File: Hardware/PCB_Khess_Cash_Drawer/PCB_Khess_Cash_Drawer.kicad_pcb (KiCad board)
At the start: 2 copper layers, 92 x 84 mm, 17 parts, among them J1 Screw_Terminal_01x02, J2 Conn_01x02, J3 RJ11_Connector, J4 USB3_A, Q1 BUK9637-100E,118, U1 R-78B5.0-2.0

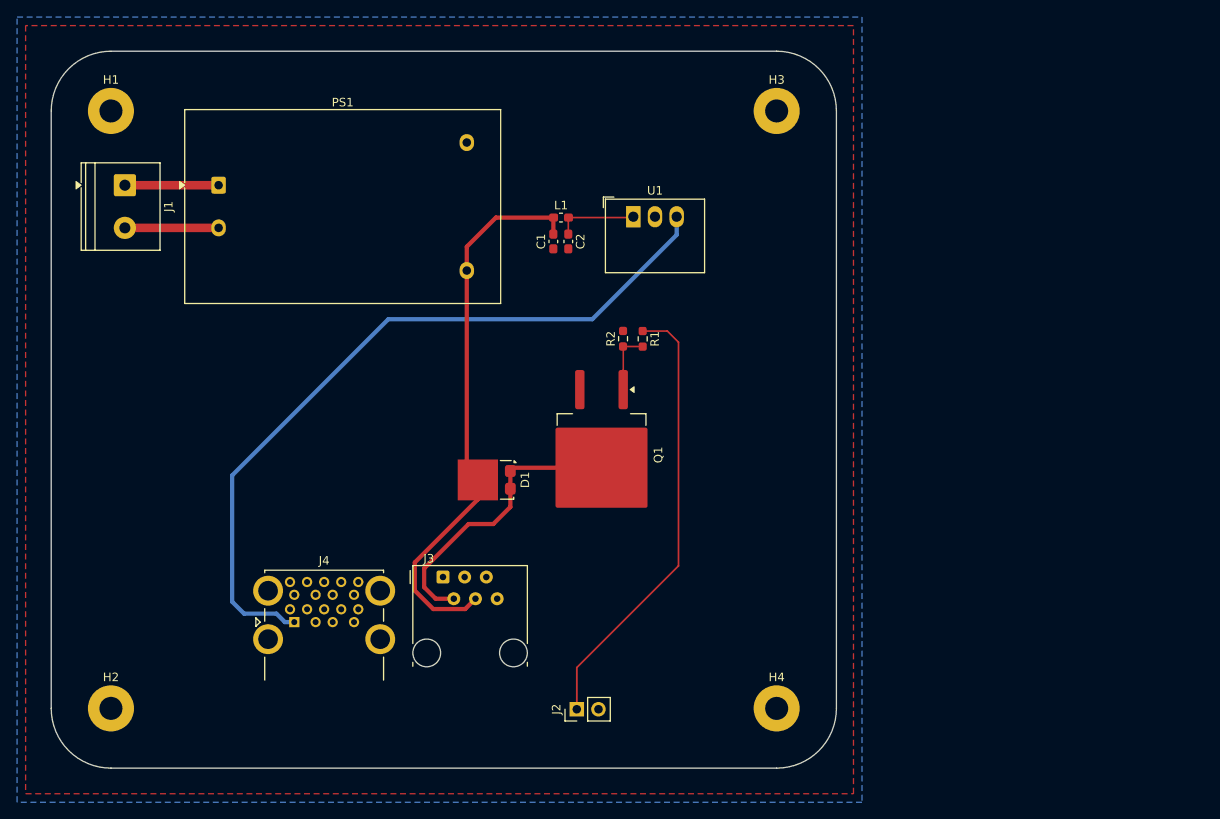
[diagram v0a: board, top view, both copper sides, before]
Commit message: fix: fix pcb
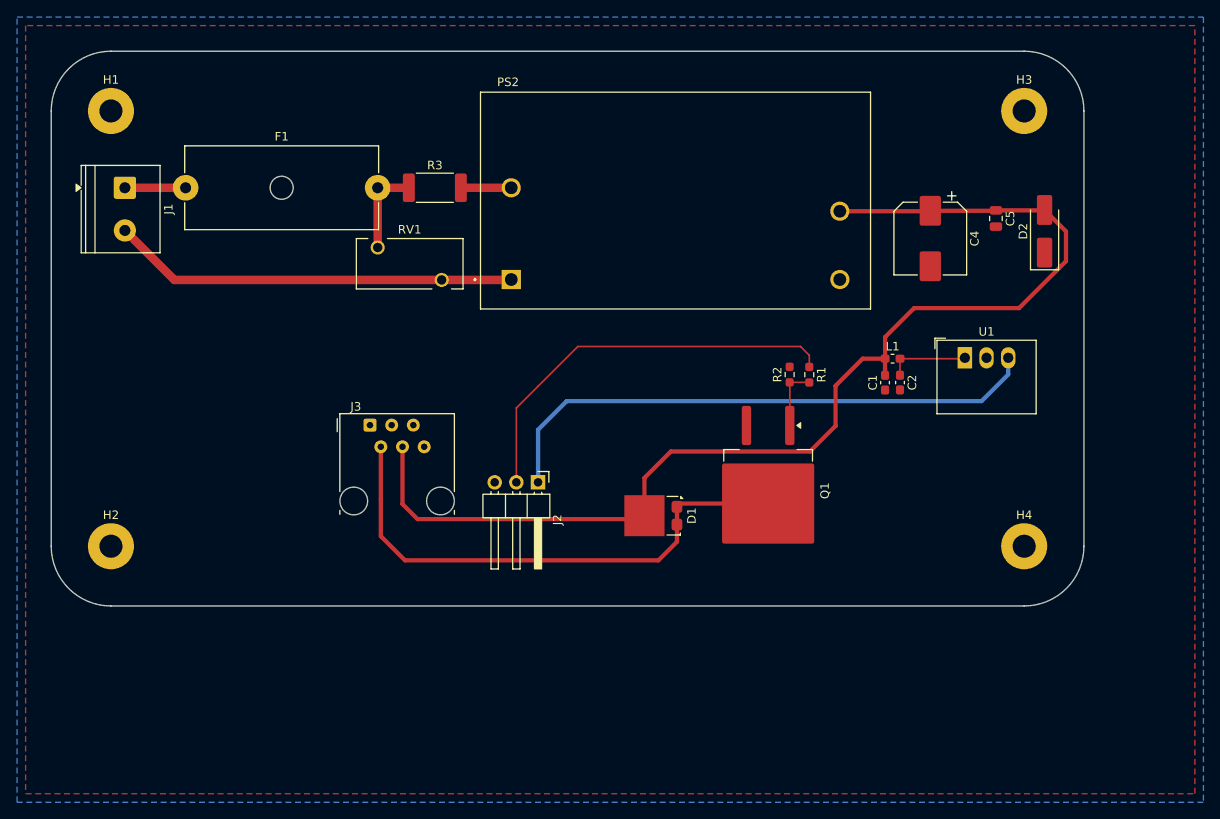
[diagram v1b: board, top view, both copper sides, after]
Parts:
- removed J4: USB3_A, Connector_USB:USB3_A_Molex_48406-0001_Horizontal_Stacked
- removed PS1: HLK-PM12, Converter_ACDC:Converter_ACDC_Hi-Link_HLK-PMxx
- added C4: 100u, Capacitor_SMD:CP_Elec_8x10, F.Cu at (176.0, 55.0)
- added C5: 1u, Capacitor_SMD:C_0805_2012Metric, F.Cu at (183.7, 52.6)
- added D2: D_TVS, Diode_SMD:D_SMA_Handsoldering, F.Cu at (189.4, 54.1)
- added F1: Fuse, Fuse:Fuseholder_Cylinder-5x20mm_Schurter_0031_8201_Horizontal_Open, F.Cu at (88.8, 49.0)
- added PS2: PSK-15E-12, PSK-15E-12:CONV_PSK-15E-12, F.Cu at (146.2, 50.5)
- added R3: 6.8, Resistor_SMD:R_2512_6332Metric_Pad1.40x3.35mm_HandSolder, F.Cu at (118.0, 49.0)
- added RV1: 10D561K, MOV-10D561K:VAR_MOV-10D561K, F.Cu at (115.0, 57.9)
- J2: value Conn_01x02 -> Conn_01x03; footprint Connector_PinHeader_2.54mm:PinHeader_1x02_P2.54mm_Vertical -> Connector_PinHeader_2.54mm:PinHeader_1x03_P2.54mm_Horizontal
- moved C1 42.2 mm to (170.7, 71.8)
- moved C2 42.2 mm to (172.4, 71.8)
- moved L1 42.2 mm to (171.6, 69.0)
- moved U1 42.2 mm to (180.1, 68.9)
- moved H4 34.7 mm to (187.0, 91.0)
- moved H3 29.0 mm to (187.0, 40.0)
- moved J2 27.0 mm to (130.0, 83.5), turned to -90 degrees
- moved D1 20.0 mm to (143.6, 87.4)
- moved Q1 20.0 mm to (157.0, 84.5)
- moved R2 20.0 mm to (159.5, 70.9)
- moved R1 20.0 mm to (161.8, 70.9)
- moved J3 19.7 mm to (110.4, 76.8)
- moved H2 19.0 mm to (80.0, 91.0)
- moved J1 0.30 mm to (81.6, 49.0)
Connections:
- net CASH_DRAWER_VCC renamed +12V
- J2 pad 1: GPIO_CONTROL -> +5V
- J2 pad 2: GND -> GPIO_CONTROL
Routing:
- net +12V: track 65.9 -> 139.9 mm
- net AC_NEUTRAL: track 11.0 -> 47.8 mm
- net CASH_DRAWER_DRIVE: track 34.9 -> 62.7 mm
- net +5V: track 89.0 -> 65.9 mm
- net AC_LINE_FUSE: track 0.00 -> 10.7 mm
- net AC_LINE_FUSE_R: track 0.00 -> 5.90 mm
- net GPIO_CONTROL: track 52.7 -> 47.8 mm
- net AC_LINE: track 11.0 -> 7.12 mm
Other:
- board size 92 x 84 mm -> 121 x 65 mm
